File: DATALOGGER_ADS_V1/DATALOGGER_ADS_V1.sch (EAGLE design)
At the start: 334 parts, among them IC1 OPA1632DR, IC10 DE10-NANO, IC11 RASPBERRY_PI_4, IC12 PCF8523, IC13 OPA1632DR, IC14 OPA1632DR, IC15 OPA1632DR, IC16 OPA1632DR, IC17 OPA1632DR, IC18 OPA1632DR, IC19 OPA1632DR, IC2 OPA1632DR, IC20 OPA1632DR, IC21 REF1004U, IC22 OPA1632DR, IC23 OPA1632DR, IC24 OPA1632DR, IC25 OPA1632DR, IC26 REF1004U, IC27 D36V28F5-5V-3.2A, IC28 D24V5F1-1.8V-500MA, IC29 D24V10F3-3.3V-1A, IC3 OPA1632DR, IC30 D24V25F5-5V-2.5A, IC31 TLV2771CDBVR, IC32 TLV2771CDBVR, IC33 TLV2771CDBVR, IC34 TLV2771CDBVR, IC35 FODM217DV, IC36 FODM217DV, IC37 FODM217DV, IC38 FODM217DV, IC39 FODM217DV, IC4 OPA1632DR, IC40 FODM217DV, IC41 FODM217DV, IC42 FODM217DV, IC5 OPA1632DR, IC6 OPA1632DR, IC7 OPA1632DR, IC8 OPA1632DR, IC9 REF1004U, J1 22-29-2021, J2 22-29-2021, J3 1985027, J4 1989764, J5 1755736, U1 OPA350EA/2K5, U2 OPA350EA/2K5, U3 ADS1178IPAPT, U4 OPA350EA/2K5, U5 OPA350EA/2K5, U6 ADS1178IPAPT, U7 OPA350EA/2K5, U8 OPA350EA/2K5, U9 ADS1178IPAPT

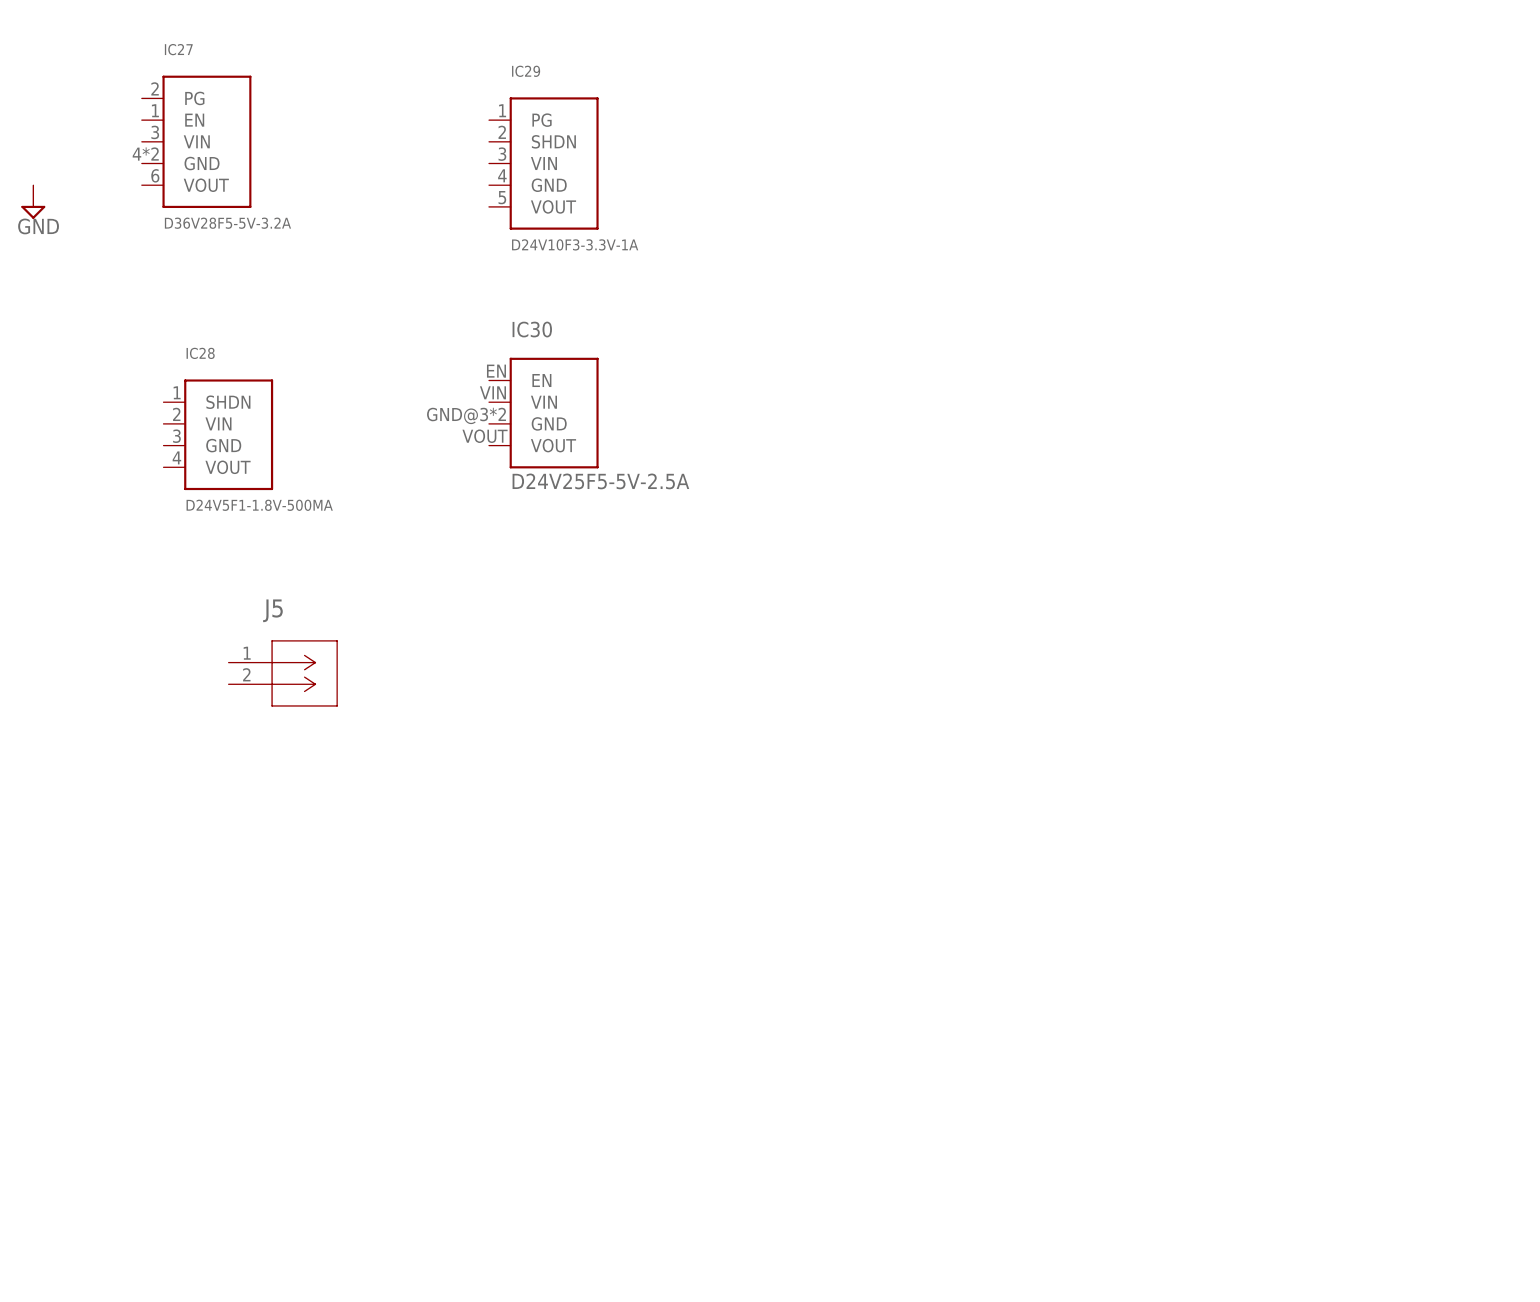
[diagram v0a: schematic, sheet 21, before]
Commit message: tarjeta_v5
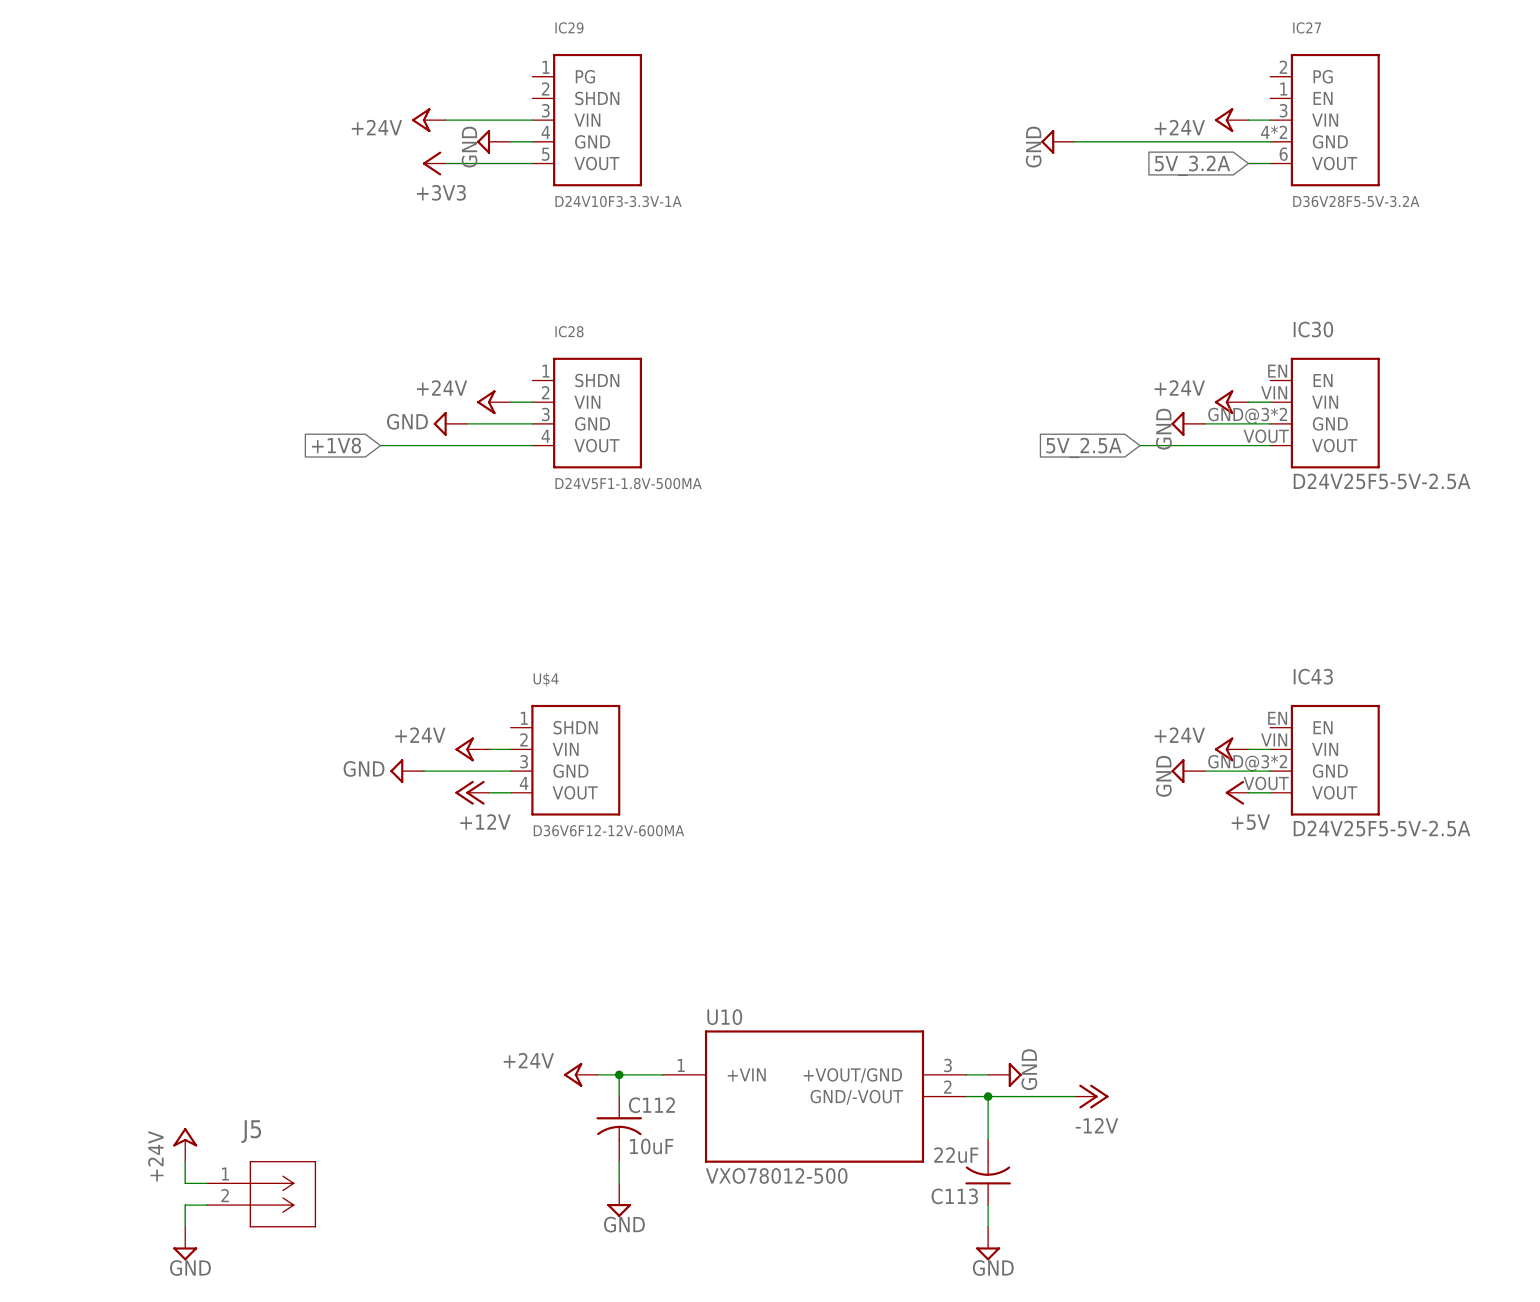
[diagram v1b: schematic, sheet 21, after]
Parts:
- added C112: 10uF, rcl:C-USC1206
- added C113: 22uF, rcl:C-USC1206
- added IC43: D24V25F5-5V-2.5A, myProyects:D24V25F5-5V-2.5A
- added U$4: D36V6F12-12V-600MA, myProyects:D36V6F12-12V-600MA
- added U10: VXO78012-500, VXO78012-500:VXO78012-500
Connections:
- new net +24V: C112.1, IC27.VIN, IC28.VIN, IC29.VIN, IC30.VIN, IC43.VIN, J5.1, U$4.VIN, U10.+VIN
- net +12V: now also U$4.VOUT
- net +1V8: now also IC28.VOUT
- net +3V3: now also IC29.VOUT
- net +5V: now also IC43.VOUT
- net -12V: now also C113.2, U10.GND/-VOUT
- net 5V_2.5A: now also IC30.VOUT
- net 5V_3.2A: now also IC27.VOUT
- net GND: now also C112.2, C113.1, IC27.GND, IC28.GND, IC29.GND, IC30.GND, IC43.GND, J5.2, U$4.GND, U10.+VOUT/GND
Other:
- moved on the sheet: IC27, IC28, IC29, IC30, J5

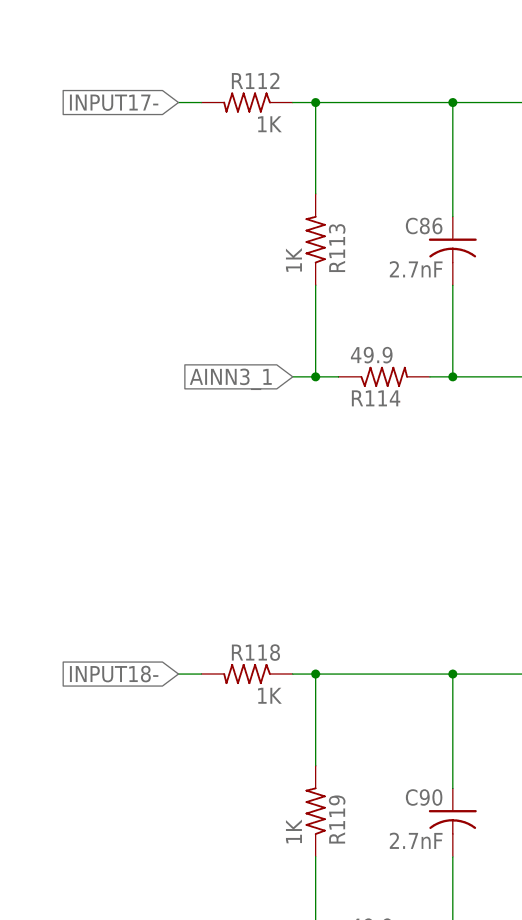
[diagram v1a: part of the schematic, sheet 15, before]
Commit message: tarjeta_v7
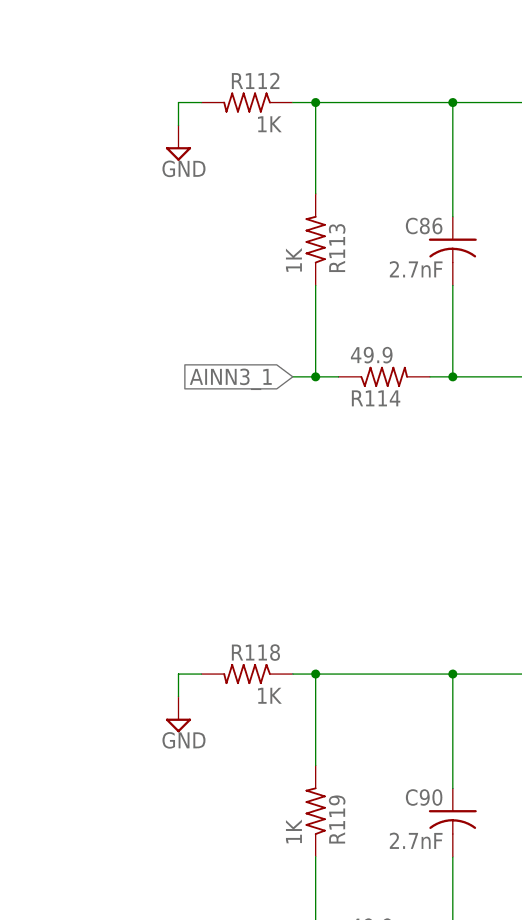
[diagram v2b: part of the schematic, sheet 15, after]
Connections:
- removed net INPUT17-: R112.2
- removed net INPUT18-: R118.2
- removed net INPUT19-: R124.2
- removed net INPUT20-: R130.2
- net GND: now also R112.2, R118.2, R124.2, R130.2
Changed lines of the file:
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@@
 <?xml version="1.0" encoding="utf-8"?>
 <!DOCTYPE eagle SYSTEM "eagle.dtd">
-<eagle version="9.5.2">
+<eagle version="9.6.2">
 <drawing>
 <settings>
@@
 <part name="SUPPLY121" library="supply2" library_urn="urn:adsk.eagle:library:372" deviceset="GND" device=""/>
 <part name="P-21" library="supply1" library_urn="urn:adsk.eagle:library:371" deviceset="-12V" device=""/>
+<part name="SUPPLY122" library="supply2" library_urn="urn:adsk.eagle:library:372" deviceset="GND" device=""/>
+<part name="SUPPLY123" library="supply2" library_urn="urn:adsk.eagle:library:372" deviceset="GND" device=""/>
+<part name="SUPPLY124" library="supply2" library_urn="urn:adsk.eagle:library:372" deviceset="GND" device=""/>
+<part name="SUPPLY125" library="supply2" library_urn="urn:adsk.eagle:library:372" deviceset="GND" device=""/>
 </parts>
 <sheets>
@@
 <attribute name="VALUE" x="72.644" y="59.309" size="1.778" layer="96" rot="MR0"/>
 </instance>
+<instance part="SUPPLY122" gate="GND" x="43.18" y="137.16" smashed="yes">
+<attribute name="VALUE" x="41.275" y="133.985" size="1.778" layer="96"/>
+</instance>
+<instance part="SUPPLY123" gate="GND" x="43.18" y="73.66" smashed="yes">
+<attribute name="VALUE" x="41.275" y="70.485" size="1.778" layer="96"/>
+</instance>
 </instances>
 <busses>
@@
 <wire x1="93.98" y1="66.04" x2="93.98" y2="63.5" width="0.1524" layer="91"/>
 </segment>
+<segment>
+<pinref part="R112" gate="G$1" pin="2"/>
+<wire x1="45.72" y1="142.24" x2="43.18" y2="142.24" width="0.1524" layer="91"/>
+<wire x1="43.18" y1="142.24" x2="43.18" y2="139.7" width="0.1524" layer="91"/>
+<pinref part="SUPPLY122" gate="GND" pin="GND"/>
+</segment>
+<segment>
+<pinref part="R118" gate="G$1" pin="2"/>
+<wire x1="45.72" y1="78.74" x2="43.18" y2="78.74" width="0.1524" layer="91"/>
+<wire x1="43.18" y1="78.74" x2="43.18" y2="76.2" width="0.1524" layer="91"/>
+<pinref part="SUPPLY123" gate="GND" pin="GND"/>
+</segment>
 </net>
 <net name="N$81" class="0">
@@
 </segment>
 </net>
-<net name="INPUT17-" class="0">
-<segment>
-<pinref part="R112" gate="G$1" pin="2"/>
-<wire x1="45.72" y1="142.24" x2="43.18" y2="142.24" width="0.1524" layer="91"/>
-<label x="43.18" y="142.24" size="1.778" layer="95" rot="MR0" xref="yes"/>
-</segment>
-</net>
 <net name="INPUT17+" class="0">
 <segment>
@@
 </segment>
 </net>
-<net name="INPUT18-" class="0">
-<segment>
-<pinref part="R118" gate="G$1" pin="2"/>
-<wire x1="45.72" y1="78.74" x2="43.18" y2="78.74" width="0.1524" layer="91"/>
-<label x="43.18" y="78.74" size="1.778" layer="95" rot="MR0" xref="yes"/>
-</segment>
-</net>
 <net name="INPUT18+" class="0">
 <segment>
@@
 <attribute name="VALUE" x="72.644" y="59.309" size="1.778" layer="96" rot="MR0"/>
 </instance>
+<instance part="SUPPLY124" gate="GND" x="43.18" y="137.16" smashed="yes">
+<attribute name="VALUE" x="41.275" y="133.985" size="1.778" layer="96"/>
+</instance>
+<instance part="SUPPLY125" gate="GND" x="43.18" y="73.66" smashed="yes">
+<attribute name="VALUE" x="41.275" y="70.485" size="1.778" layer="96"/>
+</instance>
 </instances>
 <busses>
@@
 <wire x1="93.98" y1="66.04" x2="93.98" y2="63.5" width="0.1524" layer="91"/>
 </segment>
+<segment>
+<pinref part="R124" gate="G$1" pin="2"/>
+<wire x1="45.72" y1="142.24" x2="43.18" y2="142.24" width="0.1524" layer="91"/>
+<wire x1="43.18" y1="142.24" x2="43.18" y2="139.7" width="0.1524" layer="91"/>
+<pinref part="SUPPLY124" gate="GND" pin="GND"/>
+</segment>
+<segment>
+<pinref part="R130" gate="G$1" pin="2"/>
+<wire x1="45.72" y1="78.74" x2="43.18" y2="78.74" width="0.1524" layer="91"/>
+<wire x1="43.18" y1="78.74" x2="43.18" y2="76.2" width="0.1524" layer="91"/>
+<pinref part="SUPPLY125" gate="GND" pin="GND"/>
+</segment>
 </net>
 <net name="N$89" class="0">
@@
 </segment>
 </net>
-<net name="INPUT19-" class="0">
-<segment>
-<pinref part="R124" gate="G$1" pin="2"/>
-<wire x1="45.72" y1="142.24" x2="43.18" y2="142.24" width="0.1524" layer="91"/>
-<label x="43.18" y="142.24" size="1.778" layer="95" rot="MR0" xref="yes"/>
-</segment>
-</net>
 <net name="INPUT19+" class="0">
 <segment>
@@
 </segment>
 </net>
-<net name="INPUT20-" class="0">
-<segment>
-<pinref part="R130" gate="G$1" pin="2"/>
-<wire x1="45.72" y1="78.74" x2="43.18" y2="78.74" width="0.1524" layer="91"/>
-<label x="43.18" y="78.74" size="1.778" layer="95" rot="MR0" xref="yes"/>
-</segment>
-</net>
